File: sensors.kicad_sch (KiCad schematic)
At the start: 23 parts, among them IC1 ACS724LMATR-20AB-T, IC2 ACS724LMATR-20AB-T, IC3 ACS724LMATR-20AB-T, U1 AMC1311QDWVRQ1, U6 MA732GQ-P

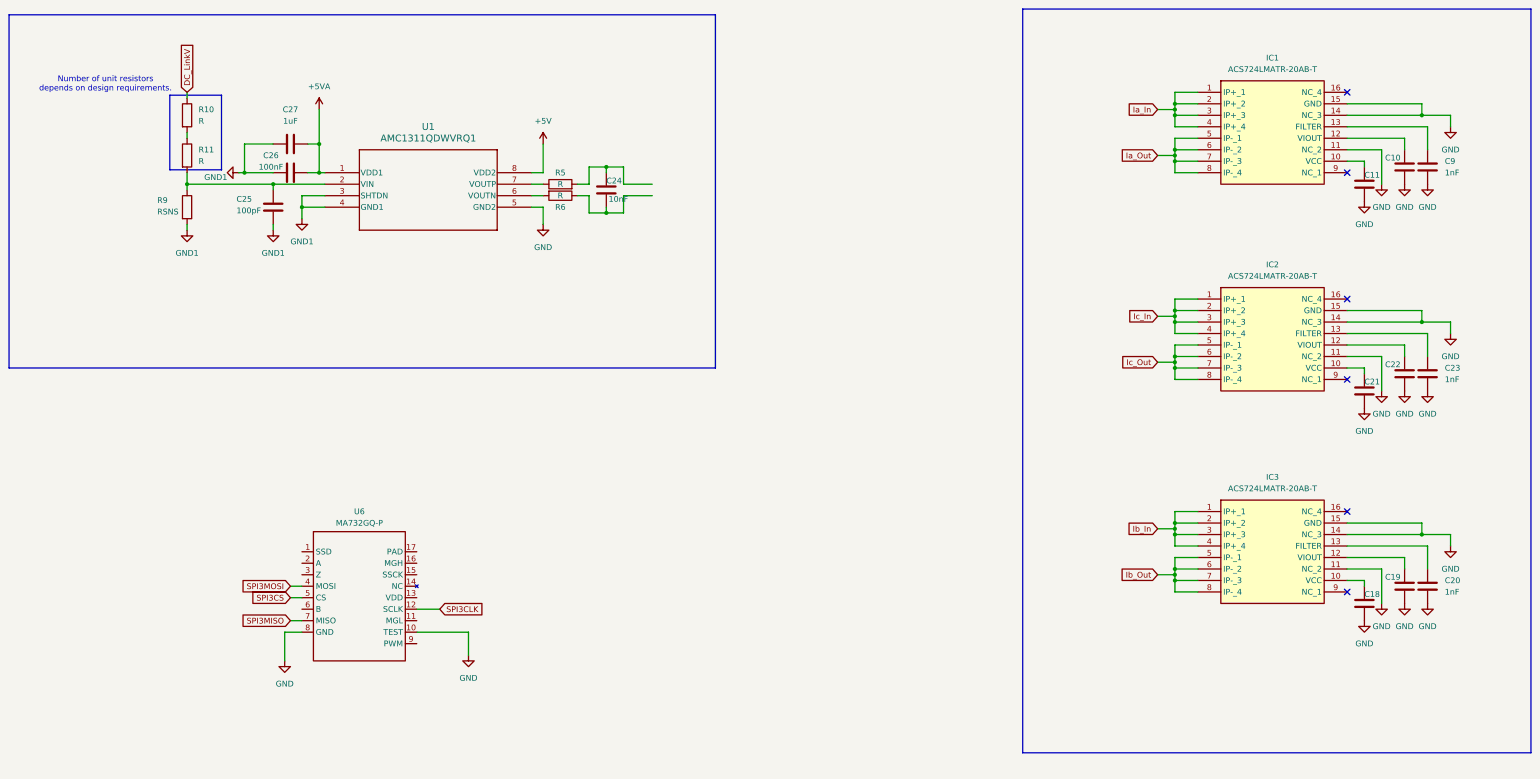
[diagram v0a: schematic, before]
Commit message: CIPOS circuit
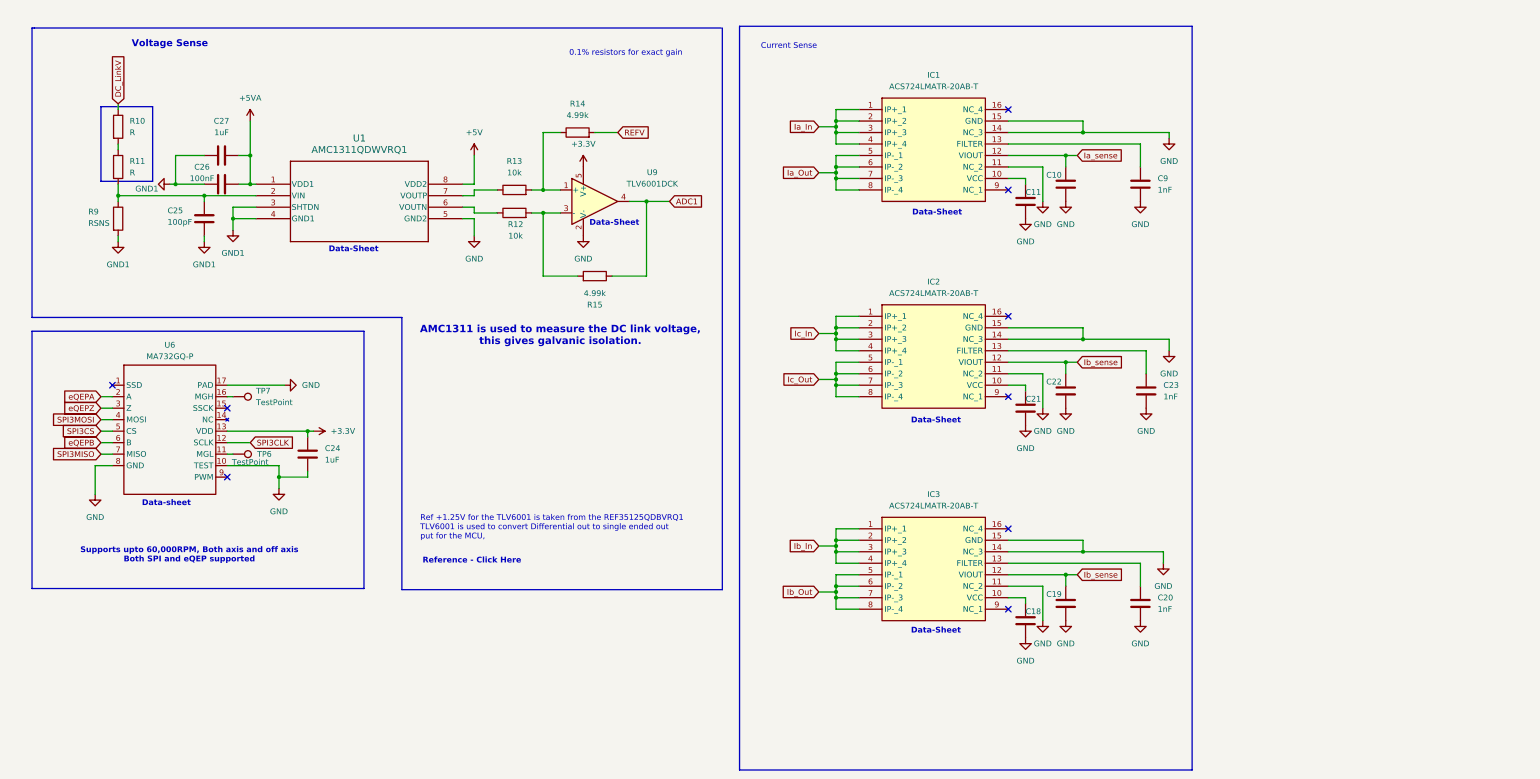
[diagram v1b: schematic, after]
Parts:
- removed R5, R6: R, symbol Device:R
- added R12, R13: 10k, symbol Device:R
- added R14, R15: 4.99k, symbol Device:R
- added TP6, TP7: TestPoint, symbol Connector:TestPoint
- added U9: TLV6001DCK, Package_TO_SOT_SMD:SOT-353_SC-70-5, symbol Amplifier_Operational:TLV6001DCK
- C24: value 10nF -> 1uF
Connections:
- net GND: now also C24.2, U6.17 (PAD), U9.2 (V-)
- net Ib_sense: now reaches C19.1, IC3.12 (VIOUT)
- net Ib_sense: now also C22.1, IC2.12 (VIOUT)
- net at U1.6 (VOUTN): now also R12.1
- net +3.3V: now reaches C24.1
- net +3.3V: now also U6.13 (VDD), U9.5 (V+)
- net Ia_sense: now reaches C10.1, IC1.12 (VIOUT)
- net at U1.7 (VOUTP): now also R13.1
- net at U6.11 (MGL): now also TP6.1
- net at U6.16 (MGH): now also TP7.1
- net eQEPA: now reaches U6.2 (A)
- net eQEPZ: now reaches U6.3 (Z)
- net eQEPB: now reaches U6.6 (B)
- new net: R13.2, R14.1, U9.1 (+)
- new net: R12.2, R15.2, U9.3 (-)
- new net ADC1: R15.1, U9.4
- new net REFV: R14.2
- no-connect marks 6 -> 9
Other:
- note added: "0.1% resistors for exact gain"
- note added: "AMC1311 is used to measure the DC link voltage, this gives galvanic isolation."
- note added: "Current Sense"
- note added: "Data-Sheet"
- note added: "Data-sheet"
- note added: "Ref +1.25V for the TLV6001 is taken from the REF35125QDBVRQ1 TLV6001 is used to convert Differential out to single ended out put for the MCU,"
- note added: "Reference - Click Here"
- note added: "Supports upto 60,000RPM, Both axis and off axis Both SPI and eQEP supported"
- note added: "Voltage Sense"
- note removed: "Number of unit resistors depends on design requirements."
- moved on the sheet: C10, C11, C18, C19, C20, C21, C22, C23, C25, C26, C27, C9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
